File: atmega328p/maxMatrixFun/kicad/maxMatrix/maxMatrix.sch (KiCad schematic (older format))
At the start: 14 parts, among them J1 max_matrix_8x16, Y1 16MHz

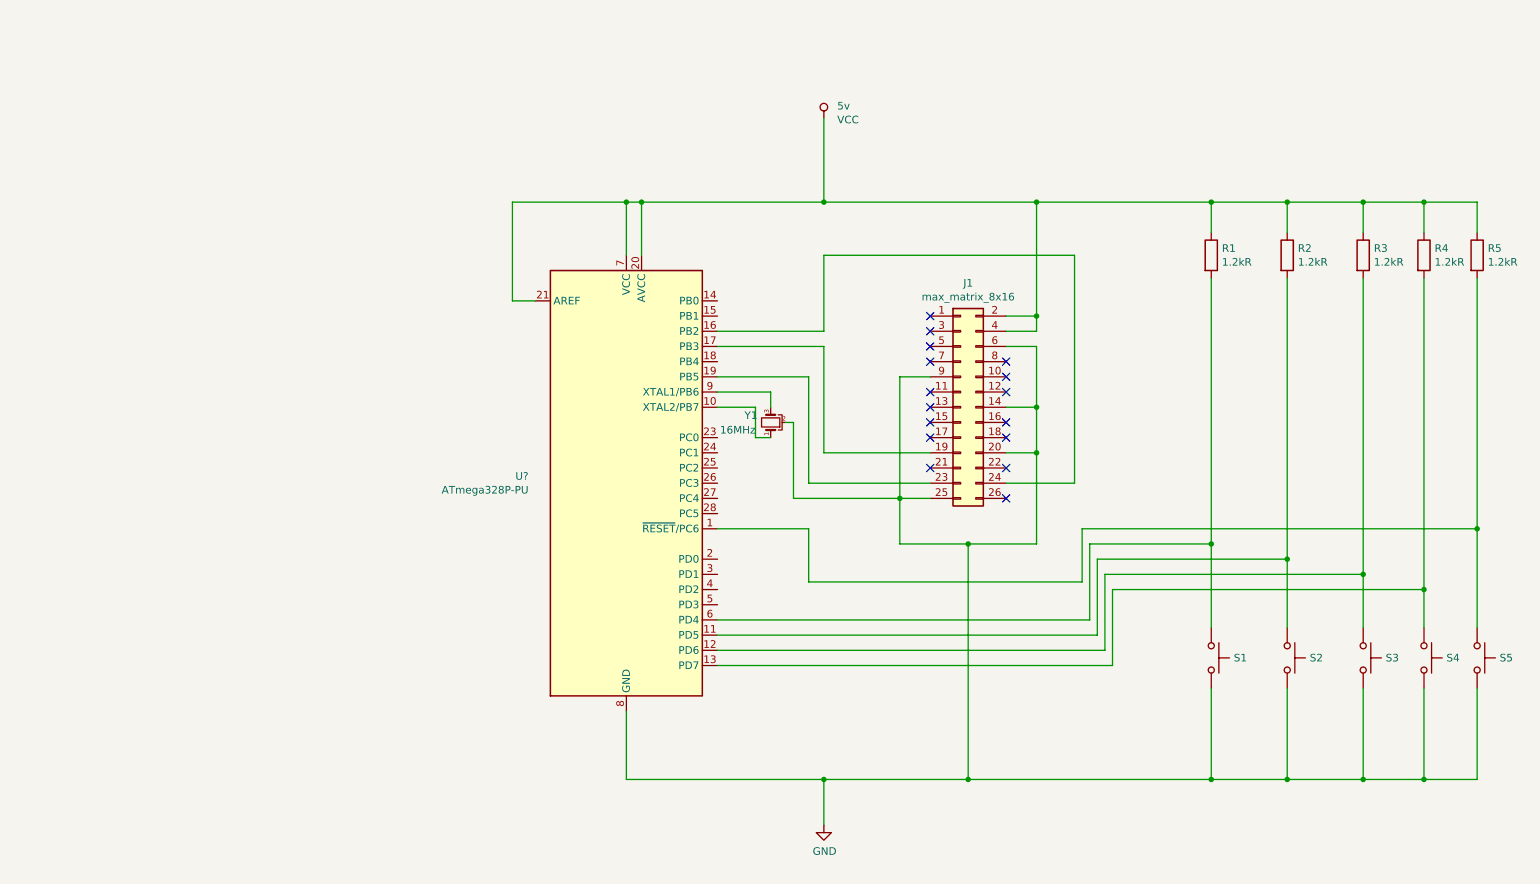
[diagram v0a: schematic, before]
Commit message: more cad
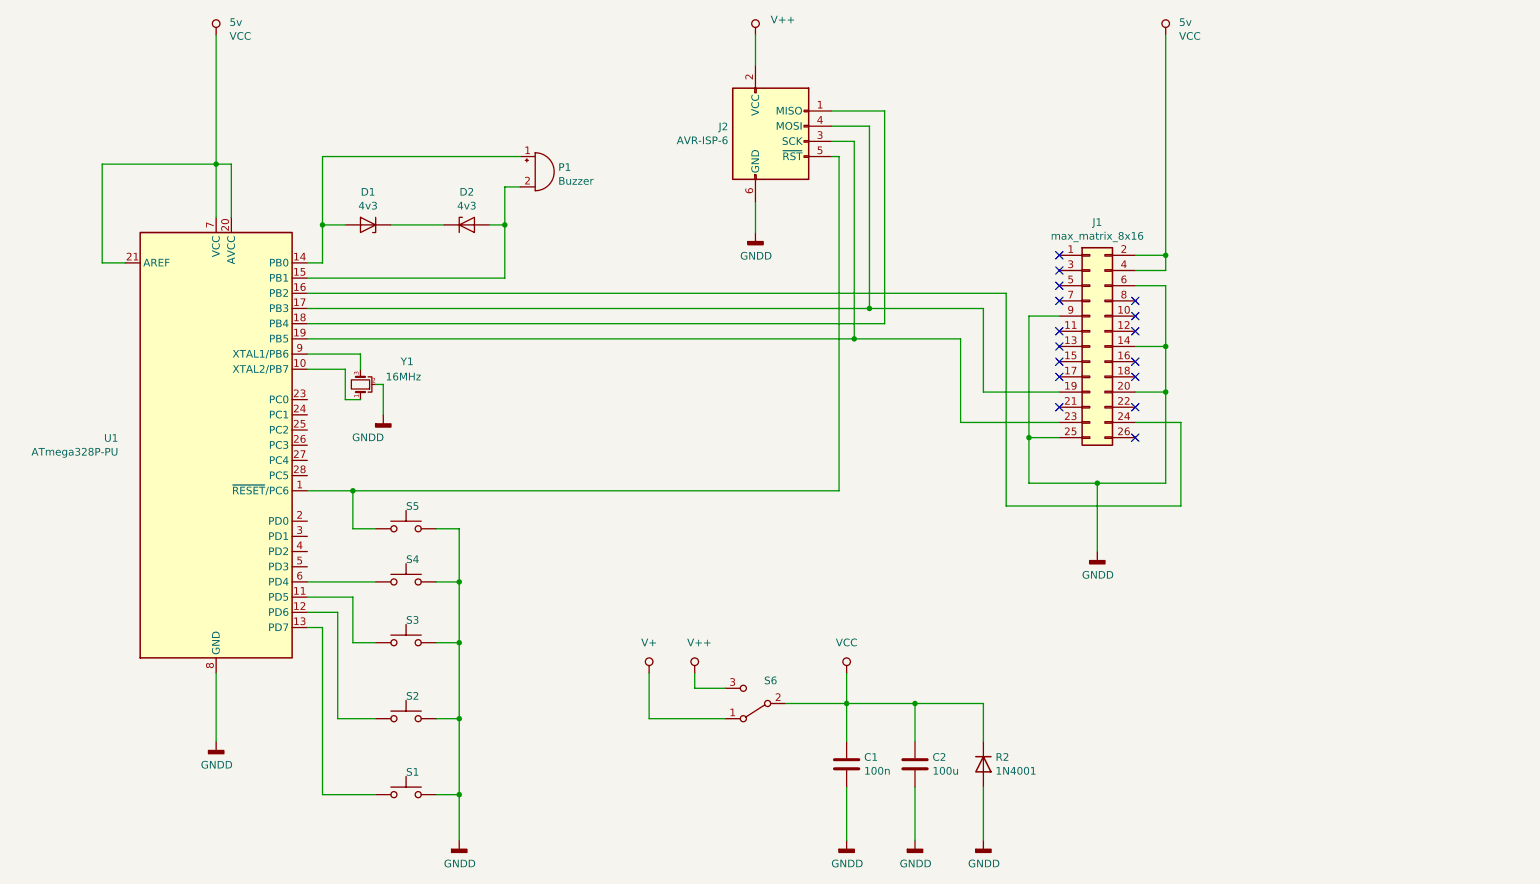
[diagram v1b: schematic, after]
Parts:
- removed R1, R2, R3, R4, R5: 1.2kR, symbol Device:R
- added 5v, V+, V++ (x2): VCC, symbol power:VCC
- added C1: 100n, symbol Device:C
- added C2: 100u, symbol Device:C
- added D1, D2: 4v3, symbol Device:D_Zener
- added J2: AVR-ISP-6, symbol Connector:AVR-ISP-6
- added P1: Buzzer, symbol Device:Buzzer
- added R2: 1N4001, symbol Simulation_SPICE:DIODE
- added S6: SW_SPDT, symbol Switch:SW_SPDT
- gave numbers to parts that had none: 1
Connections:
- net VCC: now also 5v.1 (VCC), C1.1, C2.1, J2.2 (VCC), R2.2 (K), S6.1 (A), S6.2 (B), S6.3 (C), V++.1 (VCC), V++.1 (VCC), V+.1 (VCC)
- net at S5.1, U1.1 (~RESET~/PC6): now also J2.5 (~RST)
- net at U1.11 (PD5): now also S3.1; no longer S2.1
- net at U1.12 (PD6): now also S2.1; no longer S3.1
- net at U1.13 (PD7): now also S1.1; no longer S4.1
- net at U1.14 (PB0): now also D1.2 (A), P1.1 (-)
- net at U1.15 (PB1): now also D2.2 (A), P1.2 (+)
- net at J1.19 (Pin_19), U1.17 (PB3): now also J2.4 (MOSI)
- net at U1.18 (PB4): now also J2.1 (MISO)
- net at J1.23 (Pin_23), U1.19 (PB5): now also J2.3 (SCK)
- net at U1.6 (PD4): now also S4.1; no longer S1.1
- net GND renamed GNDD
- net GNDD: now also C1.2, C2.2, J2.6 (GND), R2.1 (A)
- new net: D1.1 (K), D2.1 (K)
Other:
- moved on the sheet: J1, S1, S2, S3, S4, S5, U1, Y1
